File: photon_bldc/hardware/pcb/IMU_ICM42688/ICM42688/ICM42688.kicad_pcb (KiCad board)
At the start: 2 copper layers, 11 x 11 mm, 6 parts, among them J1 Conn_01x04, J3 Conn_01x03, U1 ICM-42688-P

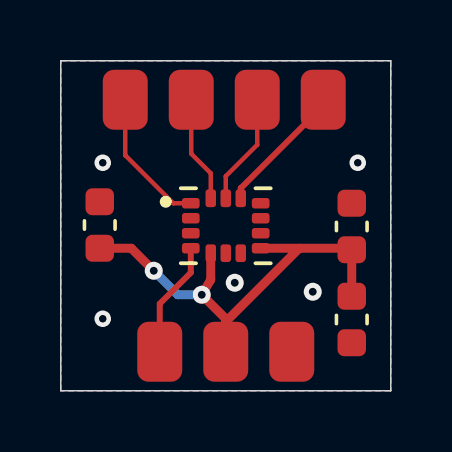
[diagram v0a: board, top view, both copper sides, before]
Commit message: SDFSDFSDF
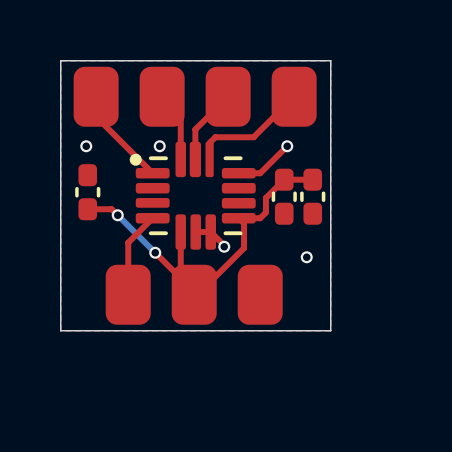
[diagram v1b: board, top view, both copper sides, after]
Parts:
- C1, C2, C3: footprint Capacitor_SMD:C_0603_1608Metric -> Capacitor_SMD:C_0402_1005Metric_Pad0.74x0.62mm_HandSolder
- moved C3 4.67 mm to (144.7, 110.7)
- moved J3 2.17 mm to (138.7, 115.2)
- moved C2 1.64 mm to (145.6, 110.7), turned to -90 degrees
- moved U1 1.41 mm to (141.7, 110.7)
- moved C1 1.16 mm to (138.1, 110.6)
- moved J1 0.98 mm to (145.8, 106.2)
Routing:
- net GND: track 0.00 -> 3.23 mm
- net +3.3V: track 16.7 -> 14.0 mm
- net SPI_MISO: track 4.77 -> 3.33 mm
- net SPI_MOSI: track 3.63 -> 2.35 mm
- net SPI_SCK: track 3.79 -> 2.54 mm
- net INT1: track 3.58 -> 2.89 mm
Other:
- board size 11 x 11 mm -> 9 x 9 mm
- board text added: "GYAT"
